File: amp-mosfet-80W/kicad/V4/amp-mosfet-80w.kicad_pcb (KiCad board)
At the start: 2 copper layers, 100.3 x 55.2 mm, 66 parts, among them J1 Conn_01x01, J2 Conn_01x01, J3 +50V, J4 -50V, J5 LS+, J6 LS-, J7 GND, Q1 BC856BS, Q11 ECX10P20, Q12 ECX10N20, Q2 BC856BS, Q3 BC846BDW1, Q4 BC846B, Q5 BC856B, Q6 DZT5551, Q7 DZT5401, Q8 BC846B

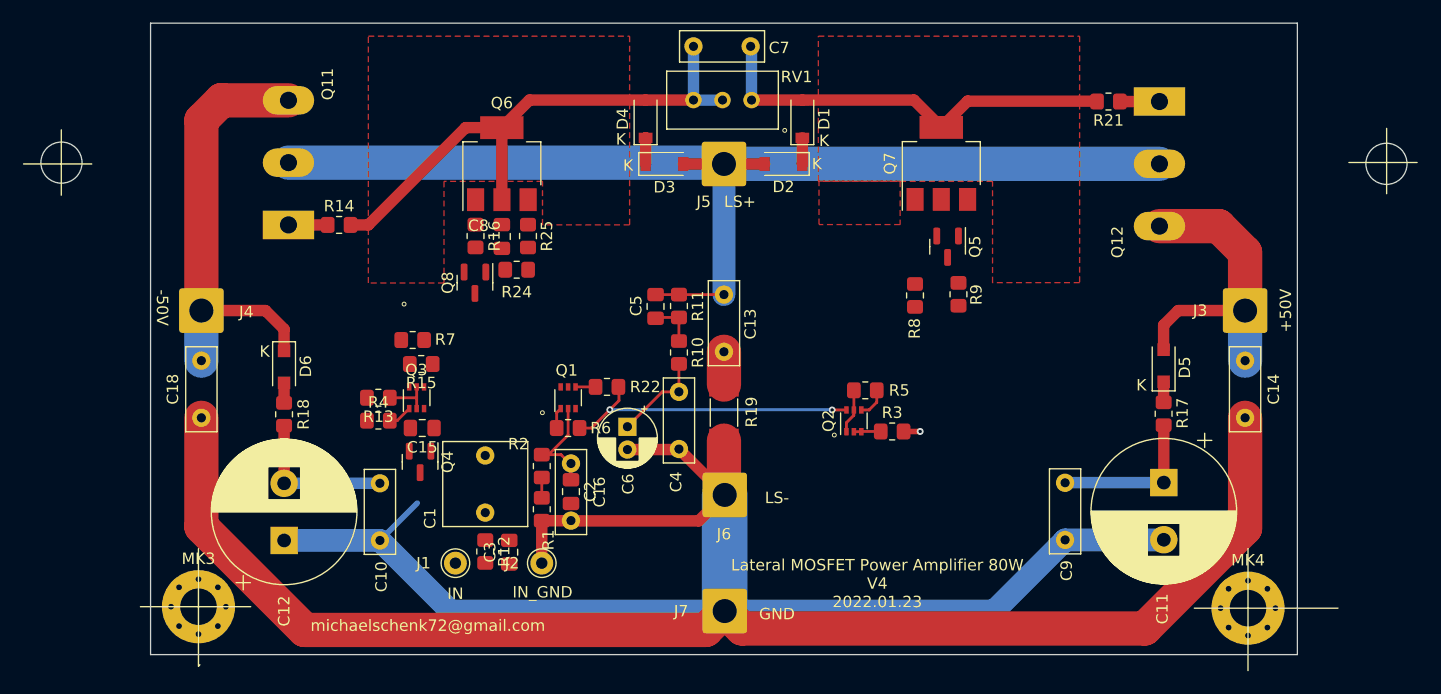
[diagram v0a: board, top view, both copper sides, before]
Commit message: Update amp-mosfet-80w.kicad_pcb
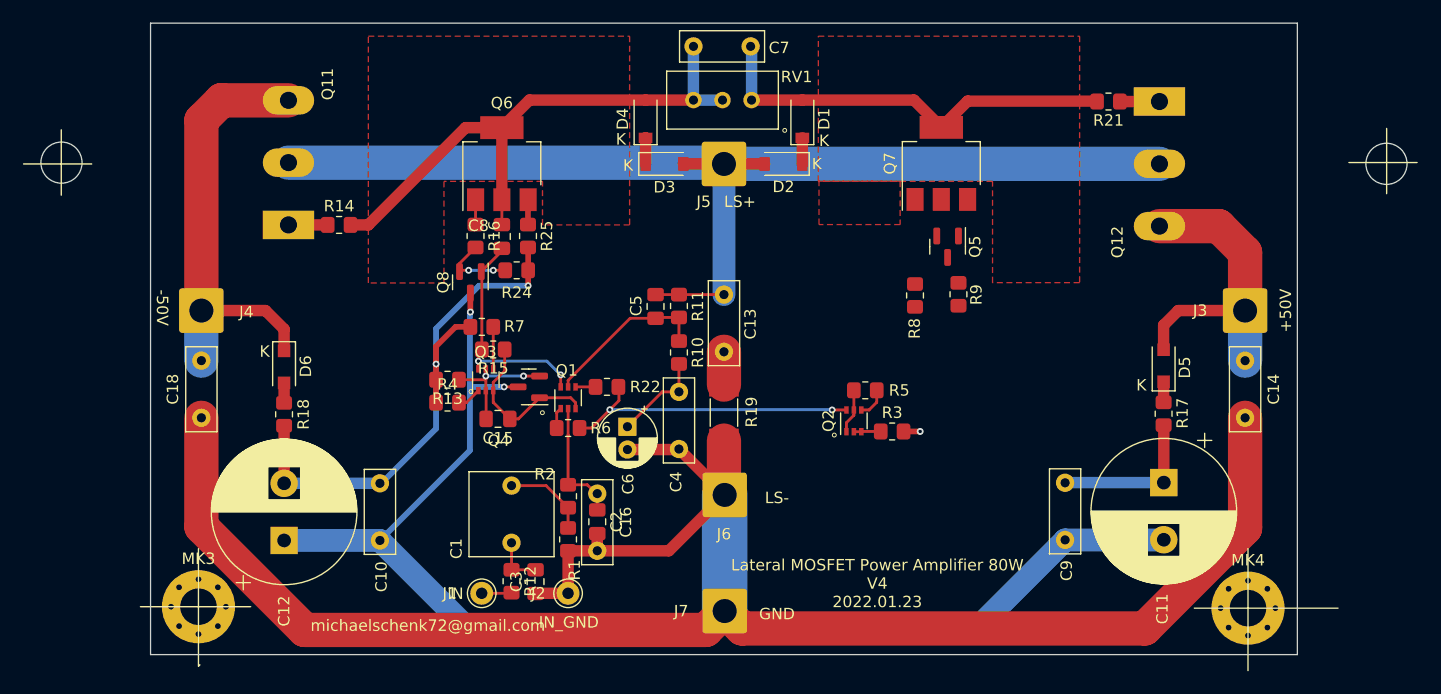
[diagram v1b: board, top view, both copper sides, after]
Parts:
- moved Q4 11.6 mm to (142.3, 76.4), turned to 180 degrees
- moved C15 6.67 mm to (139.6, 79.2)
- moved R15 6.43 mm to (139.2, 73.1)
- moved Q3 6.25 mm to (138.6, 75.8)
- moved R13 6.25 mm to (135.2, 75.8)
- moved R4 6.25 mm to (135.2, 77.8)
- moved R7 6.16 mm to (138.2, 71.2)
- moved C16 3.50 mm to (148.3, 85.7)
- moved C2 3.50 mm to (148.3, 88.2)
- moved J1 3.50 mm to (138.2, 94.5)
- moved J2 3.50 mm to (145.7, 94.5)
- moved R1 3.50 mm to (145.7, 89.7)
- moved R2 3.50 mm to (145.7, 86.0)
- moved C1 3.50 mm to (140.8, 85.0)
- moved R12 3.47 mm to (140.8, 93.4)
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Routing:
- net Net-(C10-Pad2): track 13.4 -> 50.7 mm, vias 0 -> 2
- net GND: track 253.0 -> 283.8 mm, vias 1 -> 3
- net Net-(Q1-Pad6): track 0.00 -> 20.2 mm, vias 0 -> 2
- net Net-(Q1-Pad3): track 0.00 -> 14.3 mm
- net Net-(C5-Pad2): track 4.04 -> 14.5 mm
- net Net-(Q3-Pad5): track 4.25 -> 11.4 mm, vias 0 -> 2
- net Net-(Q8-Pad2): track 0.00 -> 6.74 mm, vias 0 -> 2
- net Net-(C1-Pad1): track 1.78 -> 7.52 mm
- net Net-(C1-Pad2): track 0.00 -> 4.46 mm
- net Net-(Q3-Pad4): track 0.00 -> 3.67 mm
- net Net-(J1-Pad1): track 0.00 -> 2.63 mm
- net Net-(Q6-Pad3): track 0.00 -> 2.18 mm
- net Net-(C7-Pad1): track 48.1 -> 50.3 mm
- net Net-(Q6-Pad1): track 0.00 -> 2.18 mm
- net Net-(Q1-Pad2): track 9.62 -> 11.6 mm
